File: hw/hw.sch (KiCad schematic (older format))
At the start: 1 part

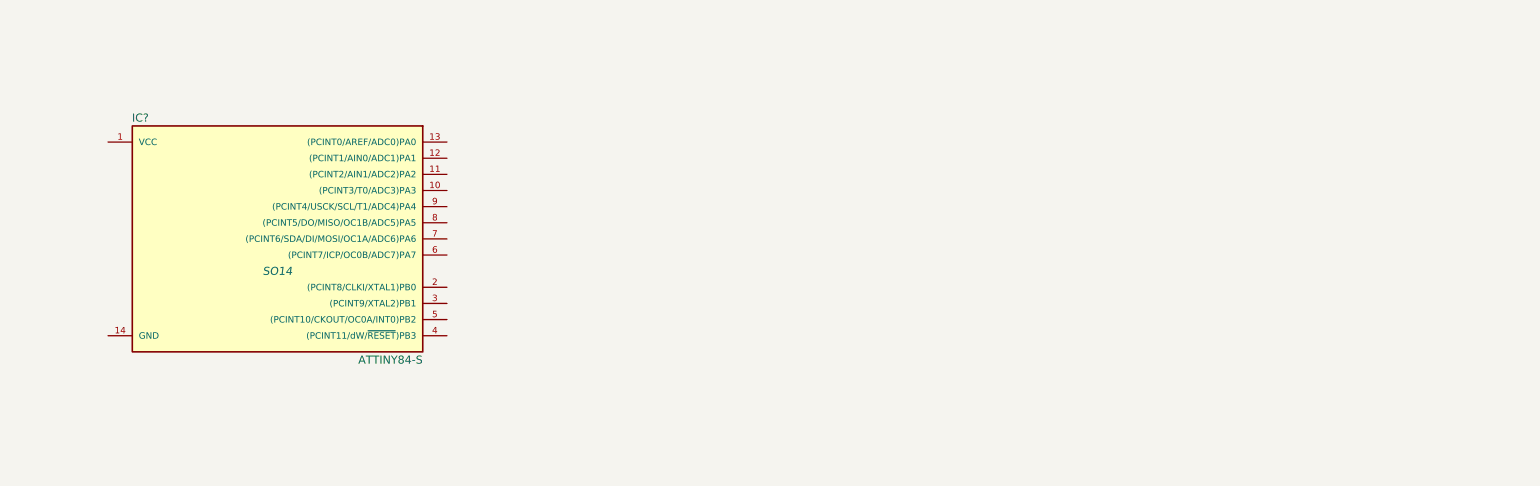
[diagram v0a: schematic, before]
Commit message: first part of board
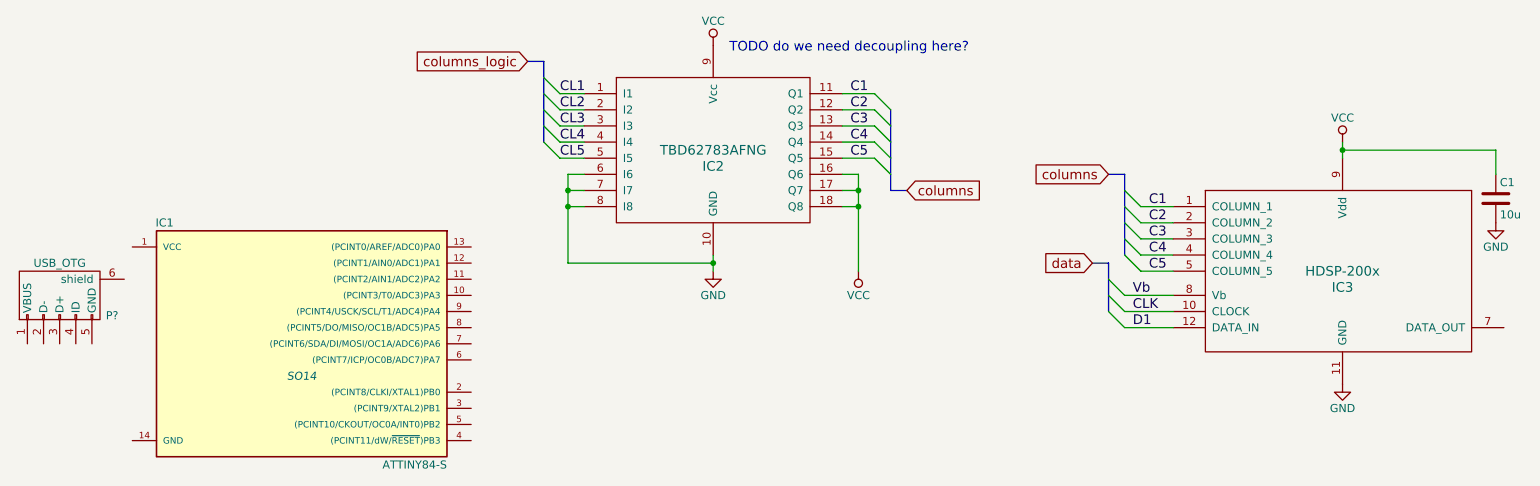
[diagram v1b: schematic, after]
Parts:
- added C1: 10u, symbol C
- added IC2: TBD62783AFNG, symbol TBD62783AFNG
- added IC3: HDSP-200x, symbol HDSP-200x
- added P?: USB_OTG, symbol USB_OTG
- gave numbers to parts that had none: 1
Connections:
- new net C1: IC2.11 (Q1), IC3.1 (COLUMN_1)
- new net C2: IC2.12 (Q2), IC3.2 (COLUMN_2)
- new net C3: IC2.13 (Q3), IC3.3 (COLUMN_3)
- new net C4: IC2.14 (Q4), IC3.4 (COLUMN_4)
- new net C5: IC2.15 (Q5), IC3.5 (COLUMN_5)
- new net CL1: IC2.1 (I1)
- new net CL2: IC2.2 (I2)
- new net CL3: IC2.3 (I3)
- new net CL4: IC2.4 (I4)
- new net CL5: IC2.5 (I5)
- new net CLK: IC3.10 (CLOCK)
- new net D1: IC3.12 (DATA_IN)
- new net GND: C1.2, IC2.10 (GND), IC2.6 (I6), IC2.7 (I7), IC2.8 (I8), IC3.11 (GND)
- new net VCC: C1.1, IC2.16 (Q6), IC2.17 (Q7), IC2.18 (Q8), IC2.9 (Vcc), IC3.9 (Vdd)
- new net Vb: IC3.8 (Vb)
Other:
- note added: "TODO do we need decoupling here?"
- moved on the sheet: IC1
